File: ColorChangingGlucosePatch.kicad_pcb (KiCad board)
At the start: 2 copper layers, 50.8 x 50.8 mm, 25 parts, among them U1 TPS76925DBVR, U2 TPS76925DBVR, U3 LMC6484, U7 CD4066BM96, U8 ATTINY204-SSFR

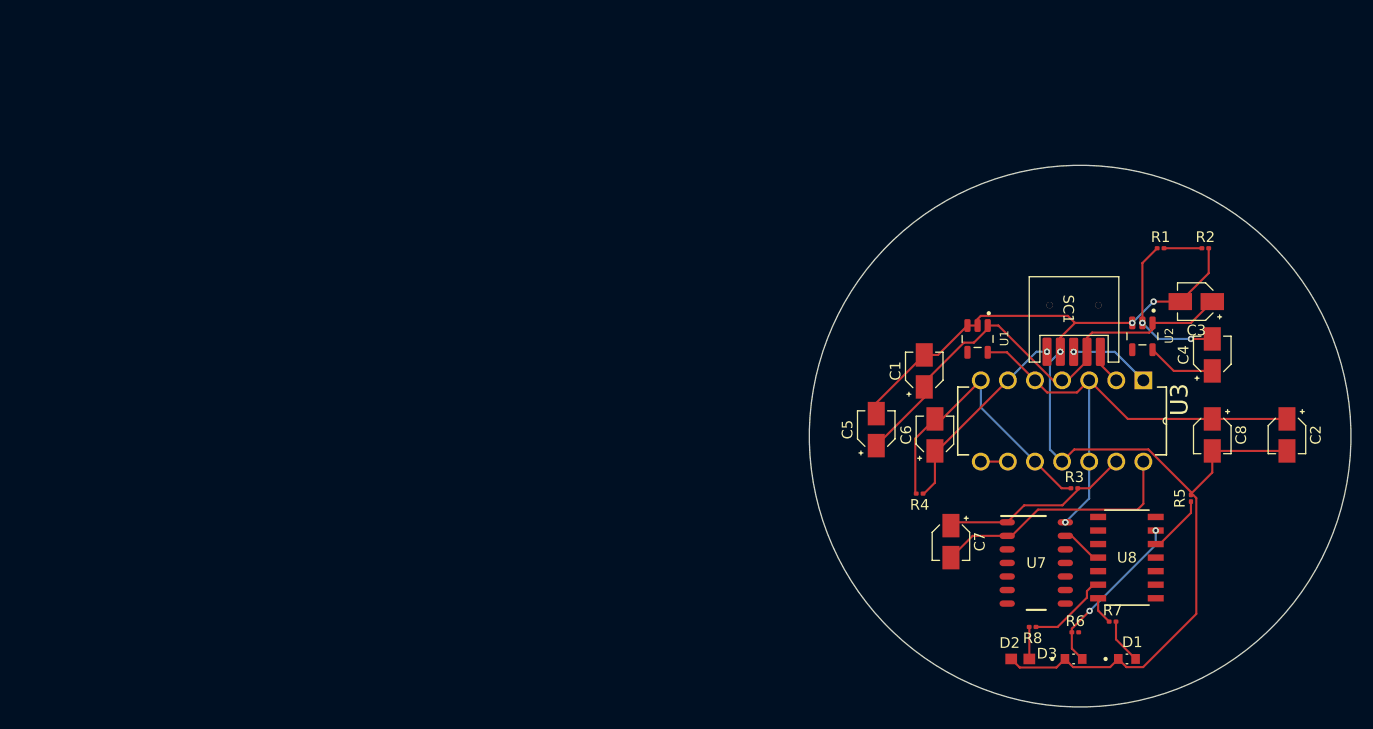
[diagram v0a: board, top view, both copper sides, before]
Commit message: final version but its not because im probably gonna work on it tomorrow.
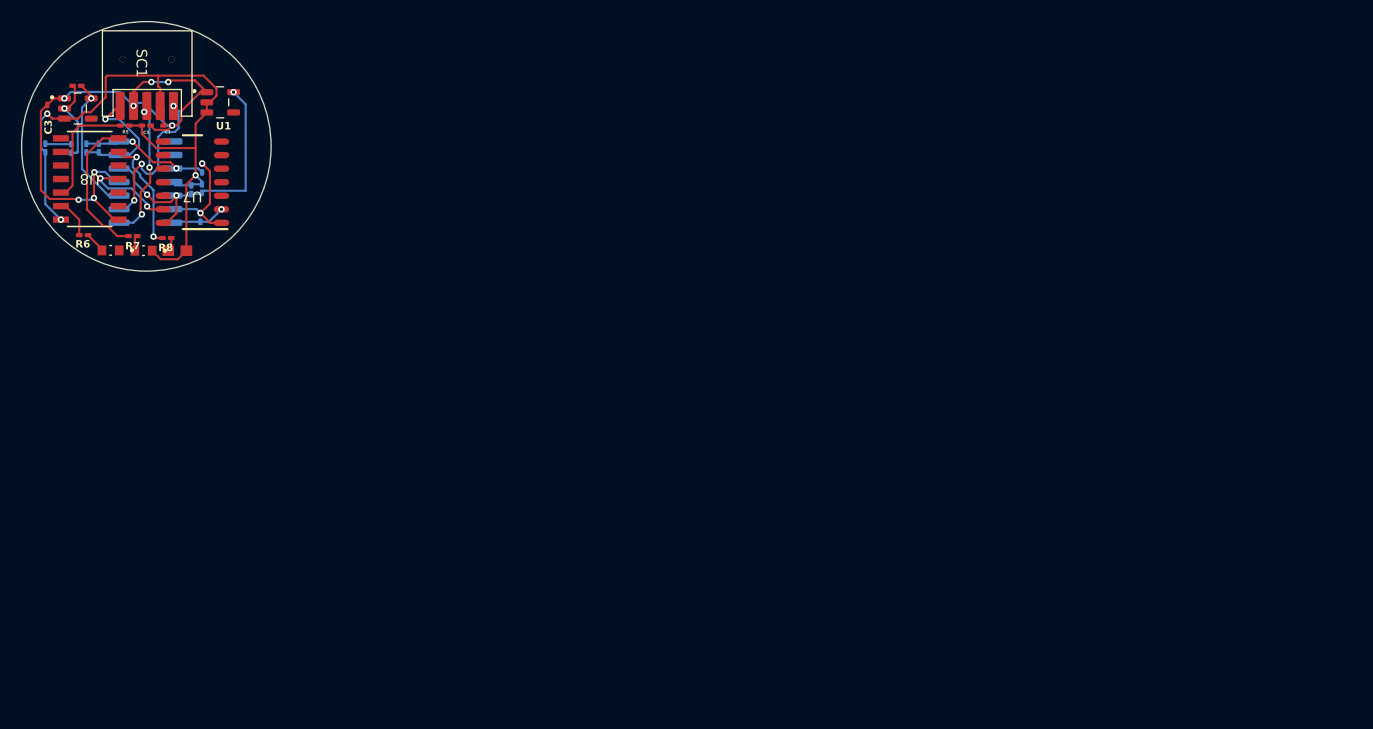
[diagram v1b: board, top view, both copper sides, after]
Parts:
- C1, C3, C4, C5: footprint Capacitor_SMD:CP_Elec_3x5.3 -> Capacitor_SMD:C_0201_0603Metric_Pad0.64x0.40mm_HandSolder
- C2, C6, C7, C8: footprint Capacitor_SMD:CP_Elec_3x5.3 -> Capacitor_SMD:C_0201_0603Metric_Pad0.64x0.40mm_HandSolder; moved to B.Cu
- R1, R2, R4: footprint Resistor_SMD:R_0201_0603Metric -> Capacitor_SMD:C_0201_0603Metric_Pad0.64x0.40mm_HandSolder; moved to B.Cu
- R3: value R_US -> 100k; footprint Resistor_SMD:R_0201_0603Metric -> Capacitor_SMD:C_0201_0603Metric_Pad0.64x0.40mm_HandSolder; moved to B.Cu
- R5: footprint Resistor_SMD:R_0201_0603Metric -> Capacitor_SMD:C_0201_0603Metric_Pad0.64x0.40mm_HandSolder
- R6, R7, R8: value R_US -> 180; footprint Resistor_SMD:R_0201_0603Metric -> Capacitor_SMD:C_0201_0603Metric_Pad0.64x0.40mm_HandSolder
- U3: footprint LMC6484AIN_NOPB-2:DIP254P762X508-14 -> LMC6484IMX_NOPB (1):SOIC127P600X175-14N; moved to B.Cu
- moved C4 109.4 mm to (76.6, 76.3), turned to 180 degrees
- moved C3 109.2 mm to (73.8, 78.5), turned to -90 degrees
- moved R2 109.1 mm to (73.6, 82.1), turned to -90 degrees
- moved R5 105.9 mm to (81.1, 80.0), turned to 0 degrees
- moved C2 105.3 mm to (87.3, 86.0), turned to 90 degrees
- moved U8 103.5 mm to (77.8, 85.0), turned to 180 degrees
- moved R1 102.5 mm to (76.0, 82.1), turned to 90 degrees
- moved U2 102.1 mm to (76.7, 78.4), turned to 0 degrees
- moved R6 100.1 mm to (77.2, 90.3)
- moved D1 99.8 mm to (82.8, 91.7), turned to 180 degrees
- moved R7 98.7 mm to (81.8, 90.4)
- moved D3 98.1 mm to (79.7, 91.7), turned to 180 degrees
- moved C8 97.5 mm to (88.3, 85.9), turned to 90 degrees
- moved SC1 89.9 mm to (83.1, 74.5)
- moved R8 89.0 mm to (85.0, 90.5), turned to 0 degrees
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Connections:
- D3 pad A: (no net) -> Net-(D3-A)
- D3 pad C: (no net) -> GND
- SC1 pad 2: +5V -> GND
- SC1 pad 4: GND -> +5V
- U3 pad 3: +2.5V -> +2.1V
- U8 pad 1: unconnected-(U8-VDD-Pad1) -> +5V
- U8 pad 14: unconnected-(U8-GND-Pad14) -> GND
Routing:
- net GND: track 113.7 -> 67.2 mm
- net Net-(U7-SIG_A_OUT_IN): track 24.1 -> 5.16 mm, vias 0 -> 1
- net +2.5V: track 45.8 -> 27.5 mm, vias 1 -> 3
- net Net-(U3C-+): track 27.6 -> 12.6 mm, vias 0 -> 2
- net Net-(SC1-Ref_Electrode): track 3.29 -> 15.4 mm, vias 0 -> 3
- net Net-(U8-PA3/EXTCLK): track 15.7 -> 3.70 mm, vias 2 -> 0
- net Net-(U8-PB2): track 2.62 -> 14.1 mm
- net +5V: track 44.0 -> 52.3 mm, vias 0 -> 8
- net Net-(U3D--): track 18.0 -> 10.5 mm, vias 0 -> 2
- net Net-(U2-GND): track 15.1 -> 8.01 mm, vias 2 -> 1
- net Net-(SC1-Wrk_Electrode): track 18.8 -> 11.8 mm
- net +2.1V: track 6.42 -> 13.1 mm, vias 0 -> 1
- net Net-(SC1-GND): track 5.48 -> 11.1 mm
- net Net-(U7-CONTROL_A): track 3.92 -> 9.10 mm, vias 0 -> 2
- net Net-(SC1-Cntr_Electrode): track 7.64 -> 12.7 mm, vias 1 -> 3
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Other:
- board size 50.8 x 50.8 mm -> 23.4 x 23.4 mm
